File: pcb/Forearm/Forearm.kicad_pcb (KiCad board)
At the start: 4 copper layers, 64 x 64.1 mm, 22 parts, among them J1 Conn_01x02, J2 Conn_01x12_Ribbon_To_Top, J3 Conn_01x12_To_Bottom, J9 Conn_01x01, U1 ESP32-S3-DEVKITC-1-N8R2, U2 4754

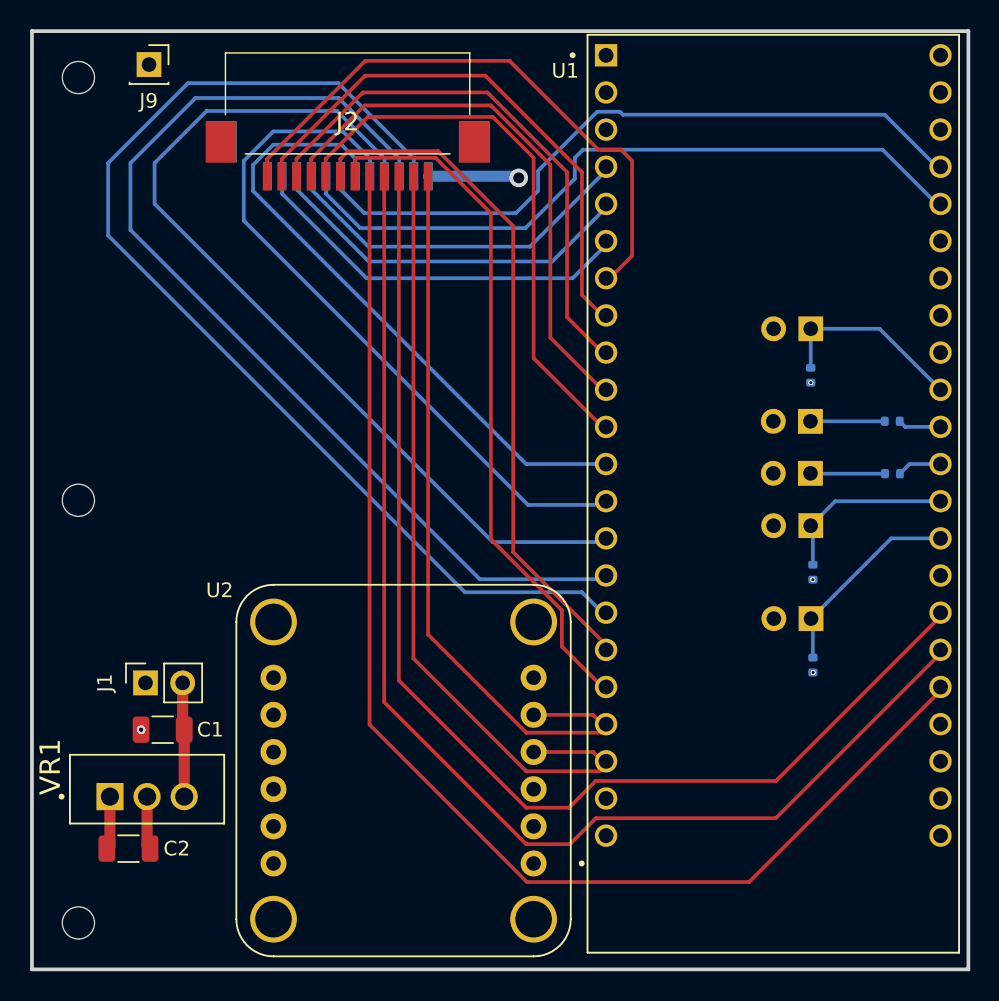
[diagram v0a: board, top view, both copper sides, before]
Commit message: revised pcbs in prep for manufacture, rev2
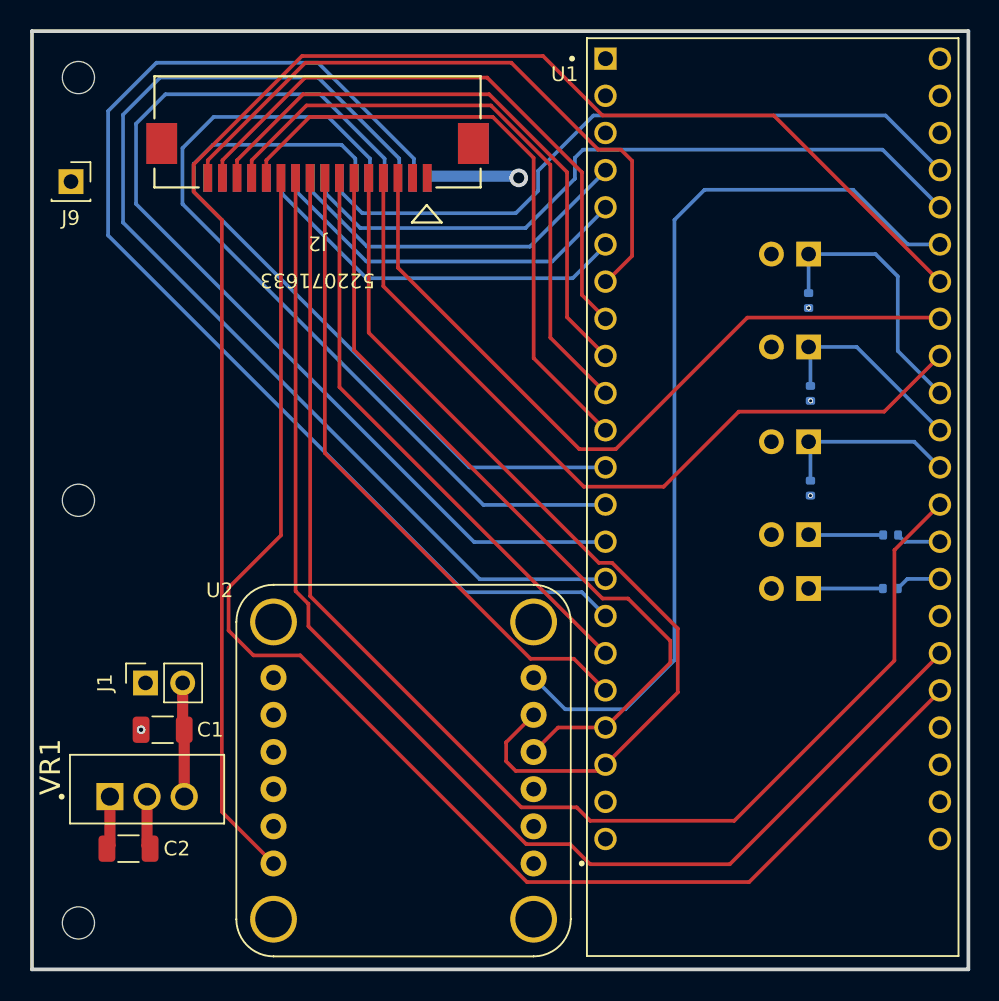
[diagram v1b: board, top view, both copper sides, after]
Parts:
- J2: value Conn_01x12_Ribbon_To_Top -> Conn_01x16_Top; footprint 0522071233:0522071233 -> 522071633:CON_522071633_MOL
- J3: value Conn_01x12_To_Bottom -> Conn_01x16_Bottom; footprint 0522071233:0522071233 -> 522071633:CON_522071633_MOL
- moved B0 18.6 mm to (65.2, 39.4)
- moved RB0 18.6 mm to (65.3, 42.5)
- moved RLED1 11.4 mm to (70.8, 55.9)
- moved LED1 11.4 mm to (65.2, 55.9)
- moved J9 9.62 mm to (14.8, 28.1)
- moved RB1 5.75 mm to (65.3, 49.0)
- moved B1 5.74 mm to (65.2, 45.8)
- moved RS0 5.11 mm to (65.2, 36.2)
- moved S0 5.11 mm to (65.2, 33.0)
- moved LED0 4.19 mm to (65.2, 52.2)
- moved RLED0 4.19 mm to (70.8, 52.2)
- moved J3 2.95 mm to (31.6, 24.6)
- moved J2 2.95 mm to (31.6, 24.6)
- moved U1 0.23 mm to (62.7, 49.6)
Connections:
- J2 pad 1: IMU_SDA -> unconnected-(J2-Pin_1-Pad1)
- J2 pad 10: FEEDBACK_D2 -> HAPTIC_S1
- J2 pad 11: FEEDBACK_D3 -> HAPTIC_S0
- J2 pad 12: FEEDBACK_D4 -> FEEDBACK_D0
- J2 pad 2: IMU_SCL -> unconnected-(J2-Pin_2-Pad2)
- J2 pad 3: HAPTIC_S2 -> IMU_1_INT
- J2 pad 4: HAPTIC_S1 -> IMU_1_RST
- J2 pad 5: HAPTIC_S0 -> IMU_SDA
- J2 pad 6: HAPTIC_SCL -> IMU_SCL
- J2 pad 7: HAPTIC_SDA -> HAPTIC_SCL
- J2 pad 8: FEEDBACK_D0 -> HAPTIC_SDA
- J2 pad 9: FEEDBACK_D1 -> HAPTIC_S2
- J3 pad 1: FREE -> unconnected-(J3-Pin_1-Pad1)
- J3 pad 10: HALL_S0 -> SPOOLPOT_ADC0
- J3 pad 11: HALL_ADC -> HALL_S3
- J3 pad 12: 3V3 -> HALL_S2
- J3 pad 2: SPOOLPOT_ADC4 -> unconnected-(J3-Pin_2-Pad2)
- J3 pad 3: SPOOLPOT_ADC3 -> unconnected-(J3-Pin_3-Pad3)
- J3 pad 4: SPOOLPOT_ADC2 -> unconnected-(J3-Pin_4-Pad4)
- J3 pad 5: SPOOLPOT_ADC1 -> unconnected-(J3-Pin_5-Pad5)
- J3 pad 6: SPOOLPOT_ADC0 -> SPOOLPOT_ADC4
- J3 pad 7: HALL_S3 -> SPOOLPOT_ADC3
- J3 pad 8: HALL_S2 -> SPOOLPOT_ADC2
- J3 pad 9: HALL_S1 -> SPOOLPOT_ADC1
- U1 pad J1_17: HAPTIC_SDA -> HAPTIC_SCL
- U1 pad J1_18: HAPTIC_SCL -> HAPTIC_SDA
- U1 pad J1_19: IMU_SDA -> IMU_SCL
- U1 pad J1_20: IMU_SCL -> IMU_SDA
- U1 pad J3_11: LED_1 -> BUTTON_0
- U1 pad J3_12: LED_0 -> BUTTON_1
- U1 pad J3_13: BUTTON_1 -> HAPTIC_S2
- U1 pad J3_14: BUTTON_0 -> LED_0
- U1 pad J3_15: unconnected-(U1-GPIO45-PadJ3_15) -> LED_1
- U1 pad J3_16: HAPTIC_S2 -> unconnected-(U1-GPIO48-PadJ3_16)
- U1 pad J3_6: unconnected-(U1-MTMS/GPIO42-PadJ3_6) -> IMU_0_INT
- U1 pad J3_7: unconnected-(U1-MTDI/GPIO41-PadJ3_7) -> IMU_0_RST
- U1 pad J3_8: unconnected-(U1-MTDO/GPIO40-PadJ3_8) -> IMU_1_INT
- U1 pad J3_9: unconnected-(U1-MTCK/GPIO39-PadJ3_9) -> IMU_1_RST
- U2 pad JP1_6: unconnected-(U2-~{INT}-PadJP1_6) -> IMU_0_INT
- U2 pad JP2_1: unconnected-(U2-BT-PadJP2_1) -> IMU_0_RST
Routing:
- net IMU_0_RST: track 0.00 -> 110.5 mm
- net IMU_0_INT: track 0.00 -> 63.1 mm
- net IMU_1_RST: track 0.00 -> 54.8 mm
- net IMU_1_INT: track 0.00 -> 52.1 mm
- net IMU_SDA: track 51.7 -> 63.2 mm
- net HAPTIC_S2: track 80.5 -> 91.4 mm
- net HALL_S2: track 48.3 -> 57.4 mm
- net HALL_S3: track 42.8 -> 51.0 mm
- net HAPTIC_SCL: track 48.0 -> 40.6 mm
- net HAPTIC_S0: track 86.4 -> 93.6 mm
- net SWITCH_0: track 13.3 -> 18.6 mm
- net HALL_S1: track 63.0 -> 68.0 mm
- net FEEDBACK_D0: track 38.5 -> 42.6 mm
- net FEEDBACK_D1: track 38.0 -> 42.1 mm
- net FEEDBACK_D3: track 37.5 -> 41.5 mm
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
